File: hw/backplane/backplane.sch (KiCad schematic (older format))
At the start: 26 parts, among them J1 out1, J10 conn5, J11 conn6, J12 out6, J2 out2, J3 conn2, J4 conn3, J5 conn1, J6 out3, J7 conn4, J8 out4, J9 out5

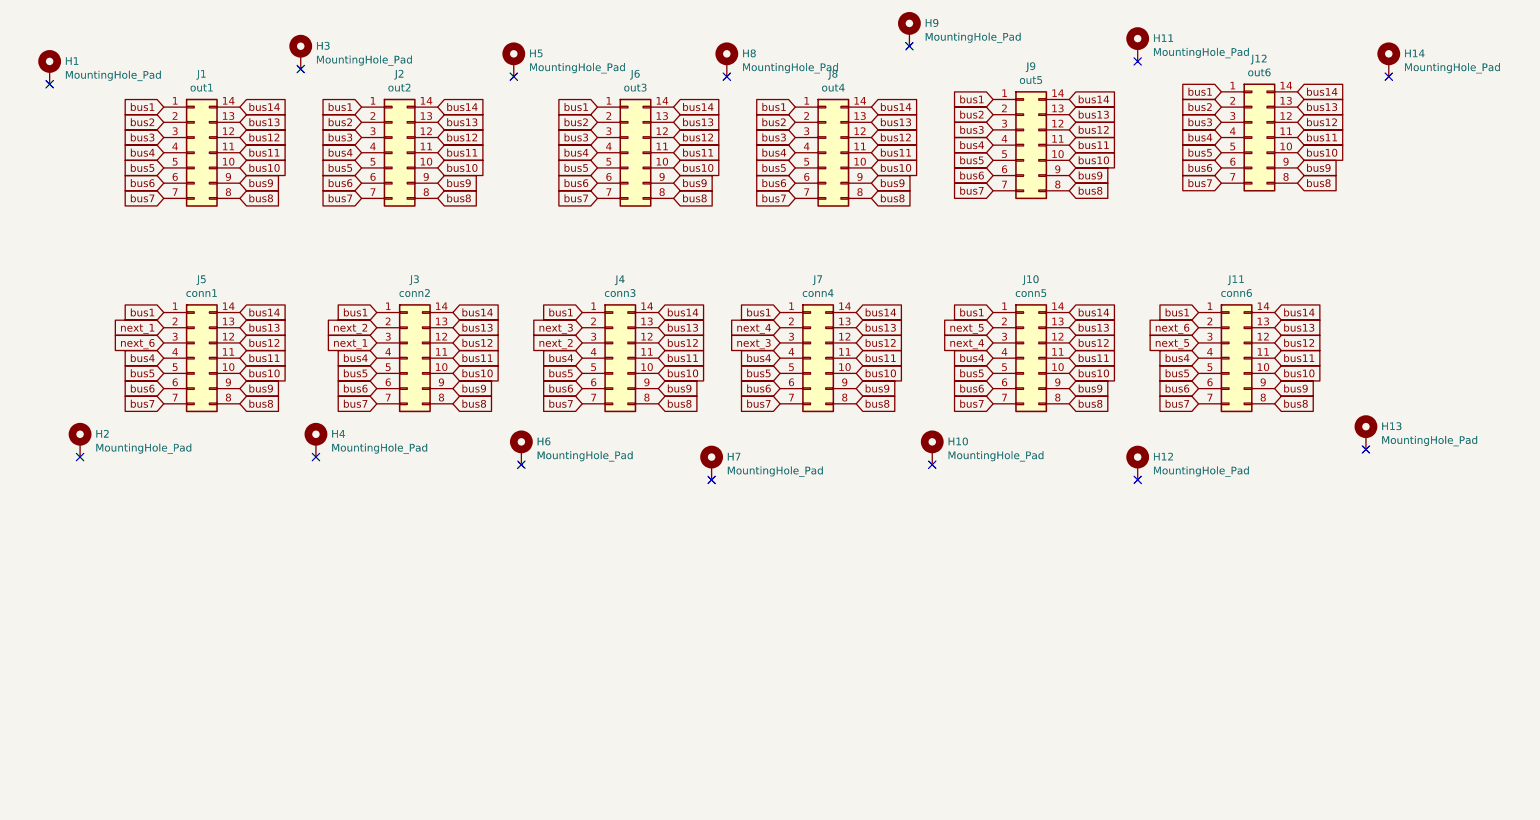
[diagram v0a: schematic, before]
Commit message: update backplane
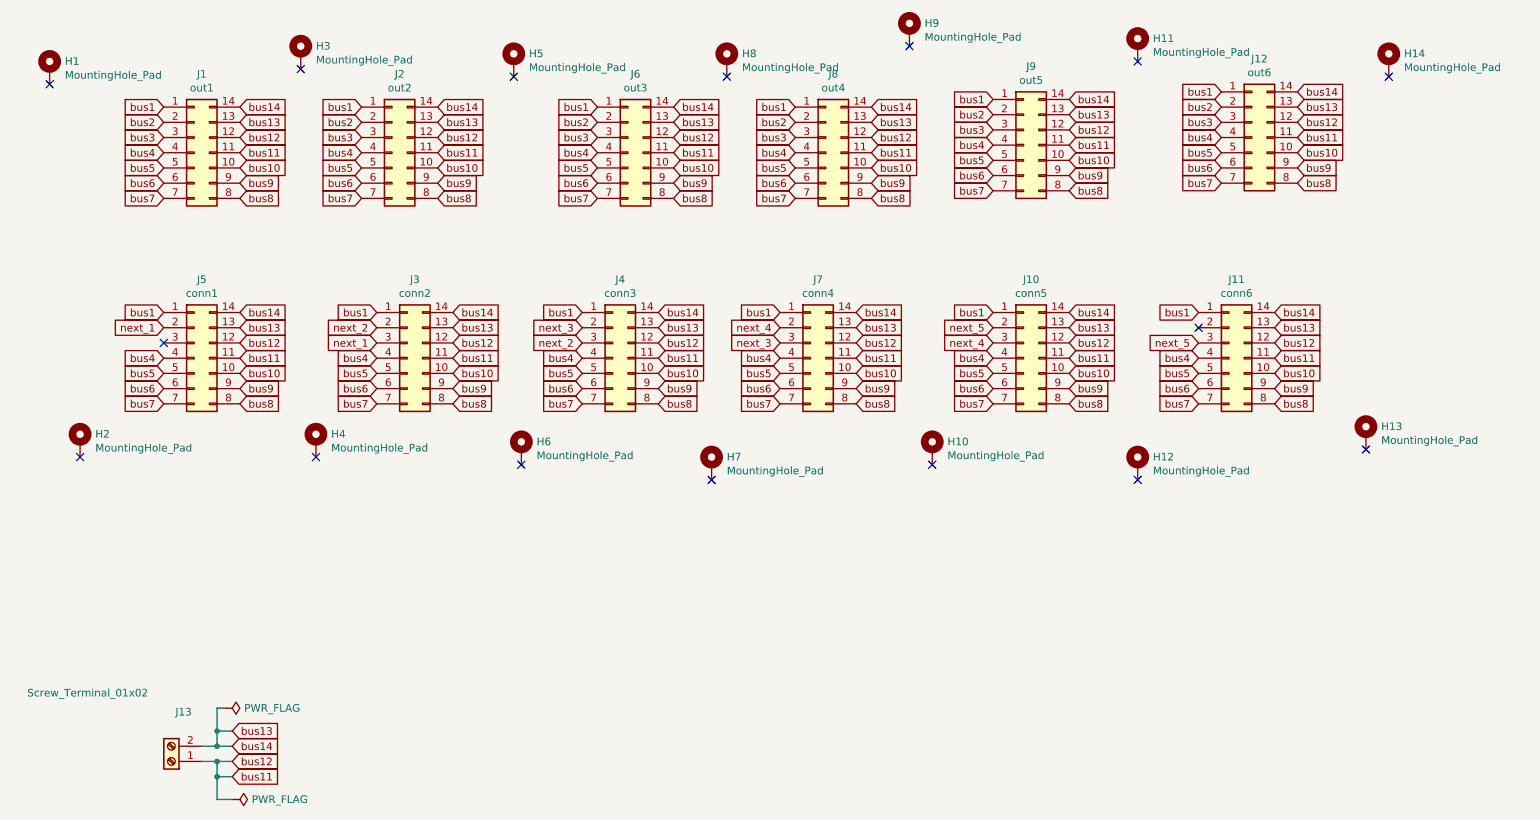
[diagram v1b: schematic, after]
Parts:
- added J13: Screw_Terminal_01x02, Connector_PinHeader_2.54mm:PinHeader_1x02_P2.54mm_Vertical, symbol Connector:Screw_Terminal_01x02
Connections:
- net bus12 is gone; now on net bus11: J1.12 (Pin_12), J10.12 (Pin_12), J11.12 (Pin_12), J12.12 (Pin_12), J2.12 (Pin_12), J3.12 (Pin_12), J4.12 (Pin_12), J5.12 (Pin_12), J6.12 (Pin_12), J7.12 (Pin_12), J8.12 (Pin_12), J9.12 (Pin_12)
- net bus14 is gone; now on net bus13: J1.14 (Pin_14), J10.14 (Pin_14), J11.14 (Pin_14), J12.14 (Pin_14), J2.14 (Pin_14), J3.14 (Pin_14), J4.14 (Pin_14), J5.14 (Pin_14), J6.14 (Pin_14), J7.14 (Pin_14), J8.14 (Pin_14), J9.14 (Pin_14)
- net bus11: now also J13.1 (Pin_1)
- net bus13: now also J13.2 (Pin_2)
- net next_6: no longer names the net of J5.3 (Pin_3)
- net next_6: no longer J11.2 (Pin_2)
- no-connect marks 14 -> 16
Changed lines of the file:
@@
 Text GLabel 2500 3550 0    50   Input ~ 0
 next_1
-Text GLabel 2500 3650 0    50   Input ~ 0
-next_6
 Text GLabel 2500 3750 0    50   Input ~ 0
 bus4
@@
 Text GLabel 9300 3450 0    50   Input ~ 0
 bus1
-Text GLabel 9300 3550 0    50   Input ~ 0
-next_6
 Text GLabel 9300 3650 0    50   Input ~ 0
 next_5
@@
 Text GLabel 9950 2100 2    50   Input ~ 0
 bus13
+NoConn ~ 2500 3650
+NoConn ~ 9300 3550
+$Comp
+L Connector:Screw_Terminal_01x02 J13
+U 1 1 5BFAB153
+P 2550 6400
+F 0 "J13" H 2470 6075 50  0000 C CNN
+F 1 "Screw_Terminal_01x02" H 3100 5950 50  0000 C CNN
+F 2 "Connector_PinHeader_2.54mm:PinHeader_1x02_P2.54mm_Vertical" H 2550 6400 50  0001 C CNN
+F 3 "~" H 2550 6400 50  0001 C CNN
+	1    2550 6400
+	-1   0    0    1
+$EndComp
+Text GLabel 2950 6300 2    50   Input ~ 0
+bus14
+Text GLabel 2950 6400 2    50   Input ~ 0
+bus12
+Text GLabel 2950 6500 2    50   Input ~ 0
+bus11
+Text GLabel 2950 6200 2    50   Input ~ 0
+bus13
+Wire Wire Line
+	2750 6300 2850 6300
+Wire Wire Line
+	2950 6200 2850 6200
+Wire Wire Line
+	2850 6200 2850 6300
+Connection ~ 2850 6300
+Wire Wire Line
+	2850 6300 2950 6300
+Wire Wire Line
+	2950 6400 2850 6400
+Wire Wire Line
+	2850 6400 2850 6500
+Wire Wire Line
+	2850 6500 2950 6500
+Connection ~ 2850 6400
+Wire Wire Line
+	2850 6400 2750 6400
+$Comp
+L power:PWR_FLAG #FLG02
+U 1 1 5BFABCF4
+P 2950 6650
+F 0 "#FLG02" H 2950 6725 50  0001 C CNN
+F 1 "PWR_FLAG" V 2950 6778 50  0000 L CNN
+F 2 "" H 2950 6650 50  0001 C CNN
+F 3 "~" H 2950 6650 50  0001 C CNN
+	1    2950 6650
+	0    1    1    0
+$EndComp
+$Comp
+L power:PWR_FLAG #FLG01
+U 1 1 5BFABD57
+P 2900 6050
+F 0 "#FLG01" H 2900 6125 50  0001 C CNN
+F 1 "PWR_FLAG" V 2900 6178 50  0000 L CNN
+F 2 "" H 2900 6050 50  0001 C CNN
+F 3 "~" H 2900 6050 50  0001 C CNN
+	1    2900 6050
+	0    1    1    0
+$EndComp
+Wire Wire Line
+	2900 6050 2850 6050
+Wire Wire Line
+	2850 6050 2850 6200
+Connection ~ 2850 6200
+Wire Wire Line
+	2850 6500 2850 6650
+Wire Wire Line
+	2850 6650 2950 6650
+Connection ~ 2850 6500
 $EndSCHEMATC
